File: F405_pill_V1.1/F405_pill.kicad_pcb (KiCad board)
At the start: 4 copper layers, 70.5 x 26.6 mm, 64 parts, among them J1 Conn_01x04_Male, J2 Conn_01x04_Male, J3 Conn_01x04_Male, J4 TYPE-C-31-M-12, J5 Conn_01x02, U1 STM32F405VGTx, U2 TJA1050T/CM,118, U3 LM1117-3.3, U4 STM32F405_pill, U5 HT7550, U6 E73-2G4M08S1C, U8 LSM6DS3, Y1 8MHz

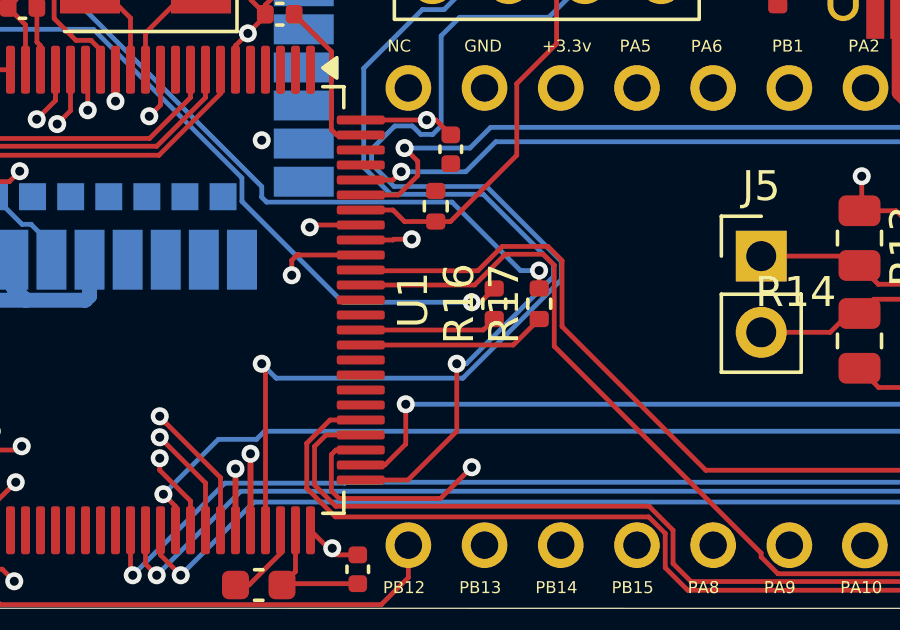
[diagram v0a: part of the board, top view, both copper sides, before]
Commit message: Fixed pin
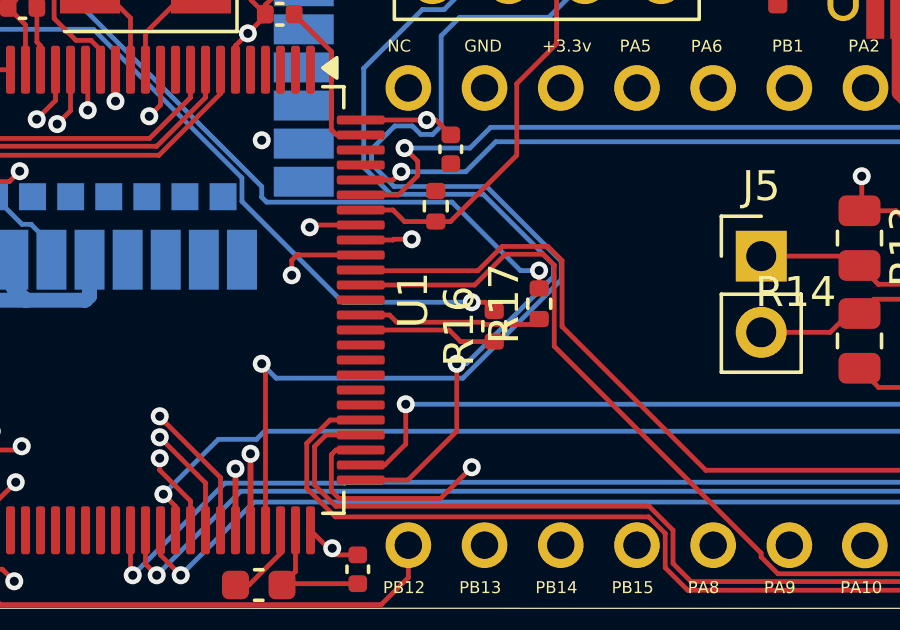
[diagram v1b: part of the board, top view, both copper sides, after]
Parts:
- moved R16 0.75 mm to (101.8, 85.0)
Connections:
- U1 pad 85: /NRF/TX -> unconnected-(U1-PD4-Pad85)
- U1 pad 87: unconnected-(U1-PD6-Pad87) -> /NRF/TX
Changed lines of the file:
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@@
 	(net 90 "unconnected-(U1-PE1-Pad98)")
 	(net 91 "unconnected-(U1-PD2-Pad83)")
-	(net 92 "unconnected-(U1-PD6-Pad87)")
+	(net 92 "unconnected-(U1-PD4-Pad85)")
 	(net 93 "unconnected-(U1-PE8-Pad39)")
 	(net 94 "unconnected-(U1-PE3-Pad2)")
@@
 			(layers "F.Cu" "F.Paste" "F.Mask")
 			(roundrect_rratio 0.25)
-			(net 15 "/NRF/TX")
+			(net 92 "unconnected-(U1-PD4-Pad85)")
 			(pinfunction "PD4")
 			(pintype "bidirectional")
@@
 			(layers "F.Cu" "F.Paste" "F.Mask")
 			(roundrect_rratio 0.25)
-			(net 92 "unconnected-(U1-PD6-Pad87)")
+			(net 15 "/NRF/TX")
 			(pinfunction "PD6")
 			(pintype "bidirectional")
@@
 	(footprint "Resistor_SMD:R_0402_1005Metric"
 		(layer "F.Cu")
-		(at 101.75 84.25 90)
+		(at 101.75 85 90)
 		(descr "Resistor SMD 0402 (1005 Metric), square (rectangular) end terminal, IPC_7351 nominal, (Body size source: IPC-SM-782 page 72, https://www.pcb-3d.com/wordpress/wp-content/uploads/ipc-sm-782a_amendment_1_and_2.pdf), generated with kicad-footprint-generator")
 		(tags "resistor")
@@
 		(tags "resistor")
 		(property "Reference" "R8"
-			(at 0 -1.17 360)
+			(at 0 -1.17 0)
 			(layer "F.SilkS")
 			(hide yes)
@@
 		)
 		(property "Value" "1k"
-			(at 0 1.17 360)
+			(at 0 1.17 0)
 			(layer "F.Fab")
 			(effects
@@
 		)
 		(property "Footprint" "Resistor_SMD:R_0402_1005Metric"
-			(at 0 0 360)
+			(at 0 0 0)
 			(layer "F.Fab")
 			(hide yes)
@@
 		)
 		(property "Datasheet" ""
-			(at 0 0 360)
+			(at 0 0 0)
 			(layer "F.Fab")
 			(hide yes)
@@
 		)
 		(property "Description" ""
-			(at 0 0 360)
+			(at 0 0 0)
 			(layer "F.Fab")
 			(hide yes)
@@
 		)
 		(fp_text user "${REFERENCE}"
-			(at 0 0 360)
+			(at 0 0 0)
 			(layer "F.Fab")
 			(effects
@@
 		(tags "resistor")
 		(property "Reference" "R12"
-			(at 0 -1.17 360)
+			(at 0 -1.17 0)
 			(layer "F.SilkS")
 			(hide yes)
@@
 		)
 		(property "Value" "1k"
-			(at 0 1.17 360)
+			(at 0 1.17 0)
 			(layer "F.Fab")
 			(effects
@@
 		)
 		(property "Footprint" "Resistor_SMD:R_0402_1005Metric"
-			(at 0 0 360)
+			(at 0 0 0)
 			(layer "F.Fab")
 			(hide yes)
@@
 		)
 		(property "Datasheet" ""
-			(at 0 0 360)
+			(at 0 0 0)
 			(layer "F.Fab")
 			(hide yes)
@@
 		)
 		(property "Description" ""
-			(at 0 0 360)
+			(at 0 0 0)
 			(layer "F.Fab")
 			(hide yes)
@@
 		)
 		(fp_text user "${REFERENCE}"
-			(at 0 0 360)
+			(at 0 0 0)
 			(layer "F.Fab")
 			(effects
@@
 	)
 	(segment
-		(start 101.29 84.2)
-		(end 101.75 83.74)
+		(start 101.46 84.2)
+		(end 101.75 84.49)
 		(width 0.16)
 		(layer "F.Cu")
@@
 	(segment
 		(start 101 84.2)
-		(end 101.29 84.2)
+		(end 101.46 84.2)
 		(width 0.16)
 		(layer "F.Cu")
@@
 	)
 	(segment
-		(start 101.385 85.125)
+		(start 100.245 85.125)
 		(end 97.3 85.125)
 		(width 0.16)
@@
 	)
 	(segment
-		(start 101.75 84.76)
-		(end 101.385 85.125)
+		(start 100.63 85.51)
+		(end 100.245 85.125)
 		(width 0.16)
 		(layer "F.Cu")
@@
 	)
 	(segment
-		(start 103.25 84.76)
-		(end 102.385 85.625)
+		(start 101.75 85.51)
+		(end 100.63 85.51)
+		(width 0.16)
+		(layer "F.Cu")
+		(net 14)
+	)
+	(segment
+		(start 98.5 84.865)
+		(end 98.26 84.625)
 		(width 0.16)
 		(layer "F.Cu")
@@
 	)
 	(segment
-		(start 102.385 85.625)
-		(end 97.3 85.625)
+		(start 98.26 84.625)
+		(end 97.3 84.625)
+		(width 0.16)
+		(layer "F.Cu")
+		(net 15)
+	)
+	(segment
+		(start 101.35578 84.865)
+		(end 98.5 84.865)
+		(width 0.16)
+		(layer "F.Cu")
+		(net 15)
+	)
+	(segment
+		(start 103.07 84.94)
+		(end 101.43078 84.94)
+		(width 0.16)
+		(layer "F.Cu")
+		(net 15)
+	)
+	(segment
+		(start 101.43078 84.94)
+		(end 101.35578 84.865)
+		(width 0.16)
+		(layer "F.Cu")
+		(net 15)
+	)
+	(segment
+		(start 103.25 84.76)
+		(end 103.07 84.94)
 		(width 0.16)
 		(layer "F.Cu")
